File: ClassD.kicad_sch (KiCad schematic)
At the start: 16 parts, among them J1 Conn_01x02_Pin, J2 Conn_01x02_Pin, U1 L78L09_TO92, U2 LM358

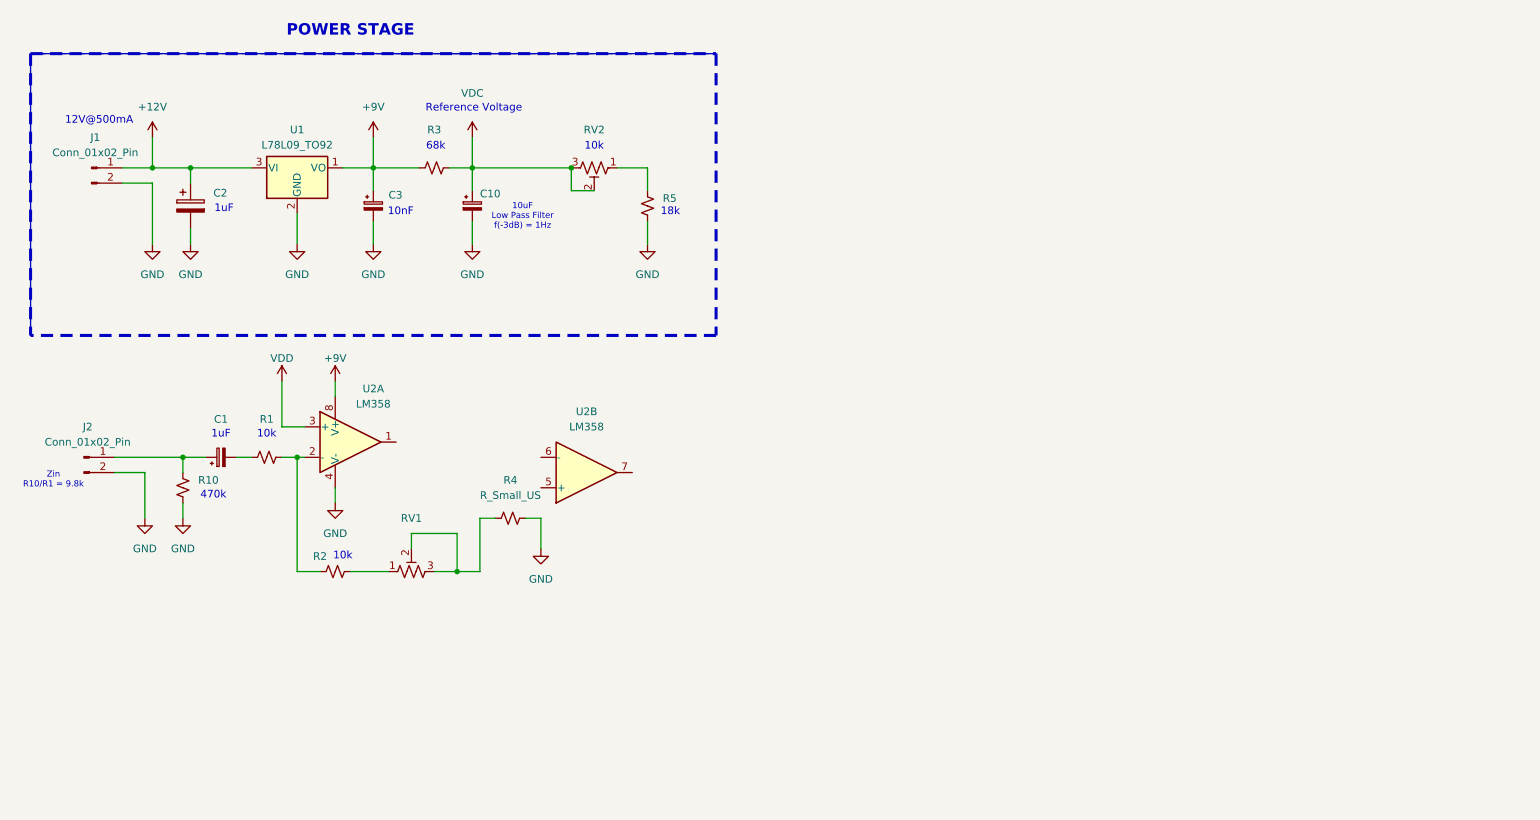
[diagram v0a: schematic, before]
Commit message: Finished Schematic Class D
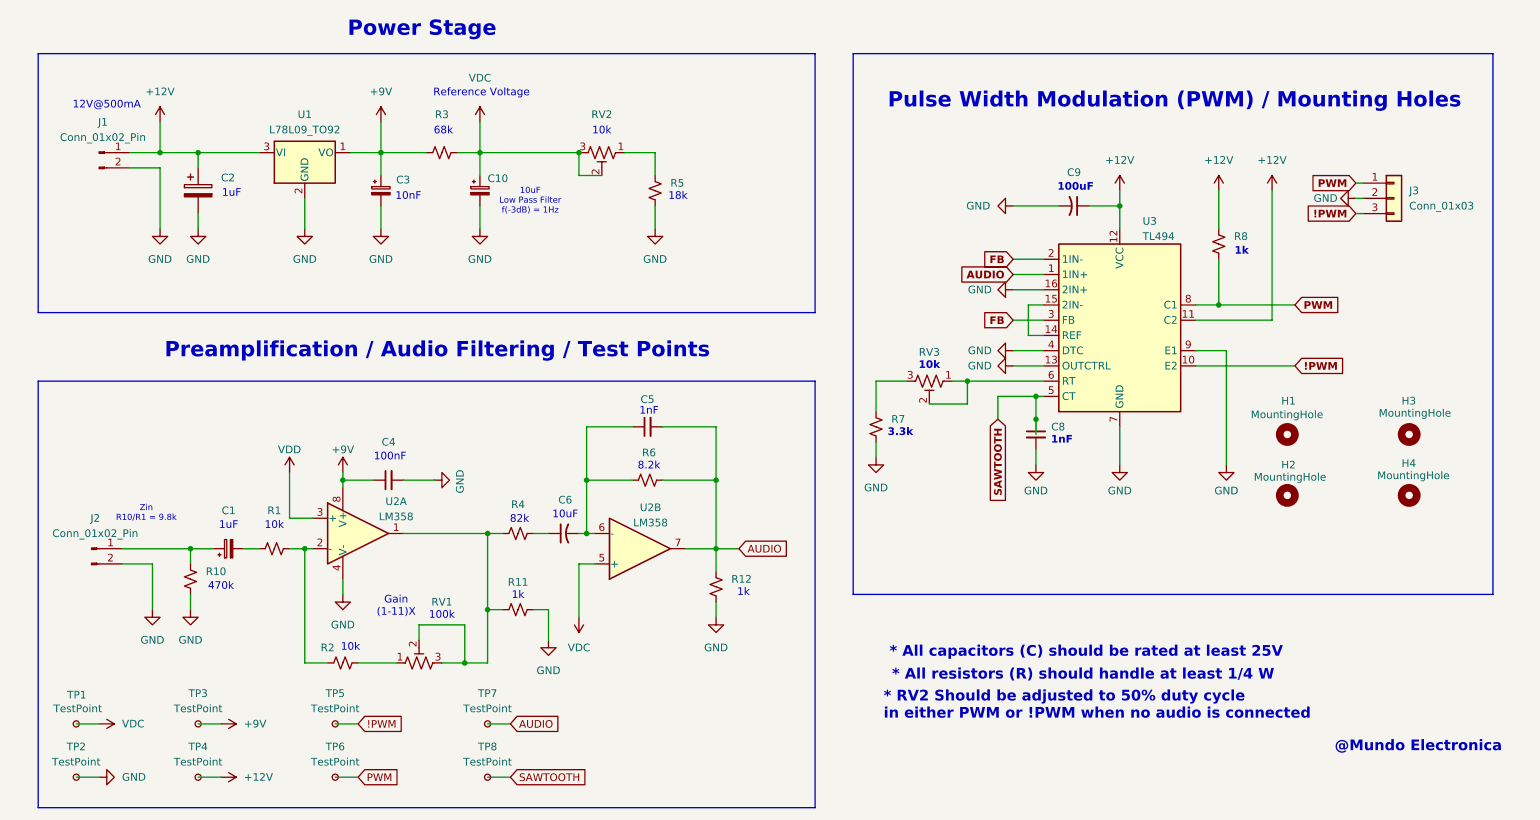
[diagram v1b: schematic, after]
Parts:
- added C4, C5, C8: C_Small, symbol Device:C_Small
- added C6, C9: C_Small_US, symbol Device:C_Small_US
- added H1, H2, H3, H4: MountingHole, symbol Mechanical:MountingHole
- added J3: Conn_01x03, symbol Connector_Generic:Conn_01x03
- added R12, R4, R6, R7, R8: R_Small_US, symbol Device:R_Small_US
- added RV3: R_Potentiometer_Trim_US, symbol Device:R_Potentiometer_Trim_US
- added TP1, TP2, TP3, TP4, TP5, TP6, TP7, TP8: TestPoint, symbol Connector:TestPoint_Small
- added U3: TL494, symbol Regulator_Controller:TL494
- renumbered R4 to R11
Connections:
- net +12V: now also C9.1, R8.1, TP4.1, U3.11 (C2), U3.12 (VCC)
- net +9V: now also C4.1, TP3.1
- net GND: now also C4.2, C8.2, C9.2, J3.2 (Pin_2), R12.2, R7.2, TP2.1, U3.13 (OUTCTRL), U3.16 (2IN+), U3.4 (DTC), U3.7 (GND), U3.9 (E1)
- net VDC: now also U2.5 (+), TP1.1
- net at R11.1, RV1.2, RV1.3: now also U2.1, R4.1
- net at U2.6 (-): now also C5.1, C6.2, R6.1
- net AUDIO: now reaches U2.7
- net AUDIO: now also C5.2, R12.1, R6.2, TP7.1, U3.1 (1IN+)
- new net: R7.1, RV3.3
- new net: C6.1, R4.2
- new net: U3.14 (REF), U3.15 (2IN-)
- new net: RV3.1, RV3.2, U3.6 (RT)
- new net !PWM: J3.3 (Pin_3), TP5.1, U3.10 (E2)
- new net FB: U3.2 (1IN-), U3.3 (FB)
- new net PWM: J3.1 (Pin_1), R8.2, TP6.1, U3.8 (C1)
- new net SAWTOOTH: C8.1, TP8.1, U3.5 (CT)
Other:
- note added: "* All capacitors (C) should be rated at least 25V"
- note added: "* All resistors (R) should handle at least 1/4 W"
- note added: "* RV2 Should be adjusted to 50% duty cycle in either PWM or !PWM when no audio is connected"
- note added: "100k"
- note added: "100nF"
- note added: "100uF"
- note added: "10uF"
- note added: "1k"
- note added: "1nF"
- note added: "3.3k"
- note added: "8.2k"
- note added: "82k"
- note added: "@Mundo Electronica"
- note added: "Gain (1-11)X"
- note added: "Power Stage"
- note added: "Preamplification / Audio Filtering / Test Points"
- note added: "Pulse Width Modulation (PWM) / Mounting Holes"
- note removed: "POWER STAGE"
- title: (none) -> ENGG220 Final Project - Victor Rosales
- moved on the sheet: C1, C10, C2, C3, J1, J2, R1, R10, R11, R2, R3, R5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
